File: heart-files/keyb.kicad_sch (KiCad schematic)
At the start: 180 parts, among them SW1 SW_Push, SW10 SW_Push, SW11 SW_Push, SW12 SW_Push, SW13 SW_Push, SW14 SW_Push, SW15 SW_Push, SW16 SW_Push, SW17 SW_Push, SW18 SW_Push, SW19 SW_Push, SW2 SW_Push, SW20 SW_Push, SW21 SW_Push, SW22 SW_Push, SW23 SW_Push, SW24 SW_Push, SW25 SW_Push, SW26 SW_Push, SW27 SW_Push, SW28 SW_Push, SW29 SW_Push, SW3 SW_Push, SW30 SW_Push, SW31 SW_Push, SW32 SW_Push, SW33 SW_Push, SW34 SW_Push, SW35 SW_Push, SW36 SW_Push, SW37 SW_Push, SW38 SW_Push, SW39 SW_Push, SW4 SW_Push, SW40 SW_Push, SW41 SW_Push, SW42 SW_Push, SW43 SW_Push, SW44 SW_Push, SW45 SW_Push, SW46 SW_Push, SW47 SW_Push, SW48 SW_Push, SW49 SW_Push, SW5 SW_Push, SW50 SW_Push, SW51 SW_Push, SW52 SW_Push, SW53 SW_Push, SW54 SW_Push, SW55 SW_Push, SW56 SW_Push, SW57 SW_Push, SW58 SW_Push, SW59 SW_Push, SW6 SW_Push, SW60 SW_Push, SW61 SW_Push, SW62 SW_Push, SW63 SW_Push, SW64 SW_Push, SW65 SW_Push, SW66 SW_Push, SW67 SW_Push, SW68 SW_Push, SW69 SW_Push, SW7 SW_Push, SW70 SW_Push, SW71 SW_Push, SW72 SW_Push, SW73 SW_Push, SW74 SW_Push, SW75 SW_Push, SW76 SW_Push, SW77 SW_Push, SW78 SW_Push, SW79 SW_Push, SW8 SW_Push, SW80 SW_Push, SW81 SW_Push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

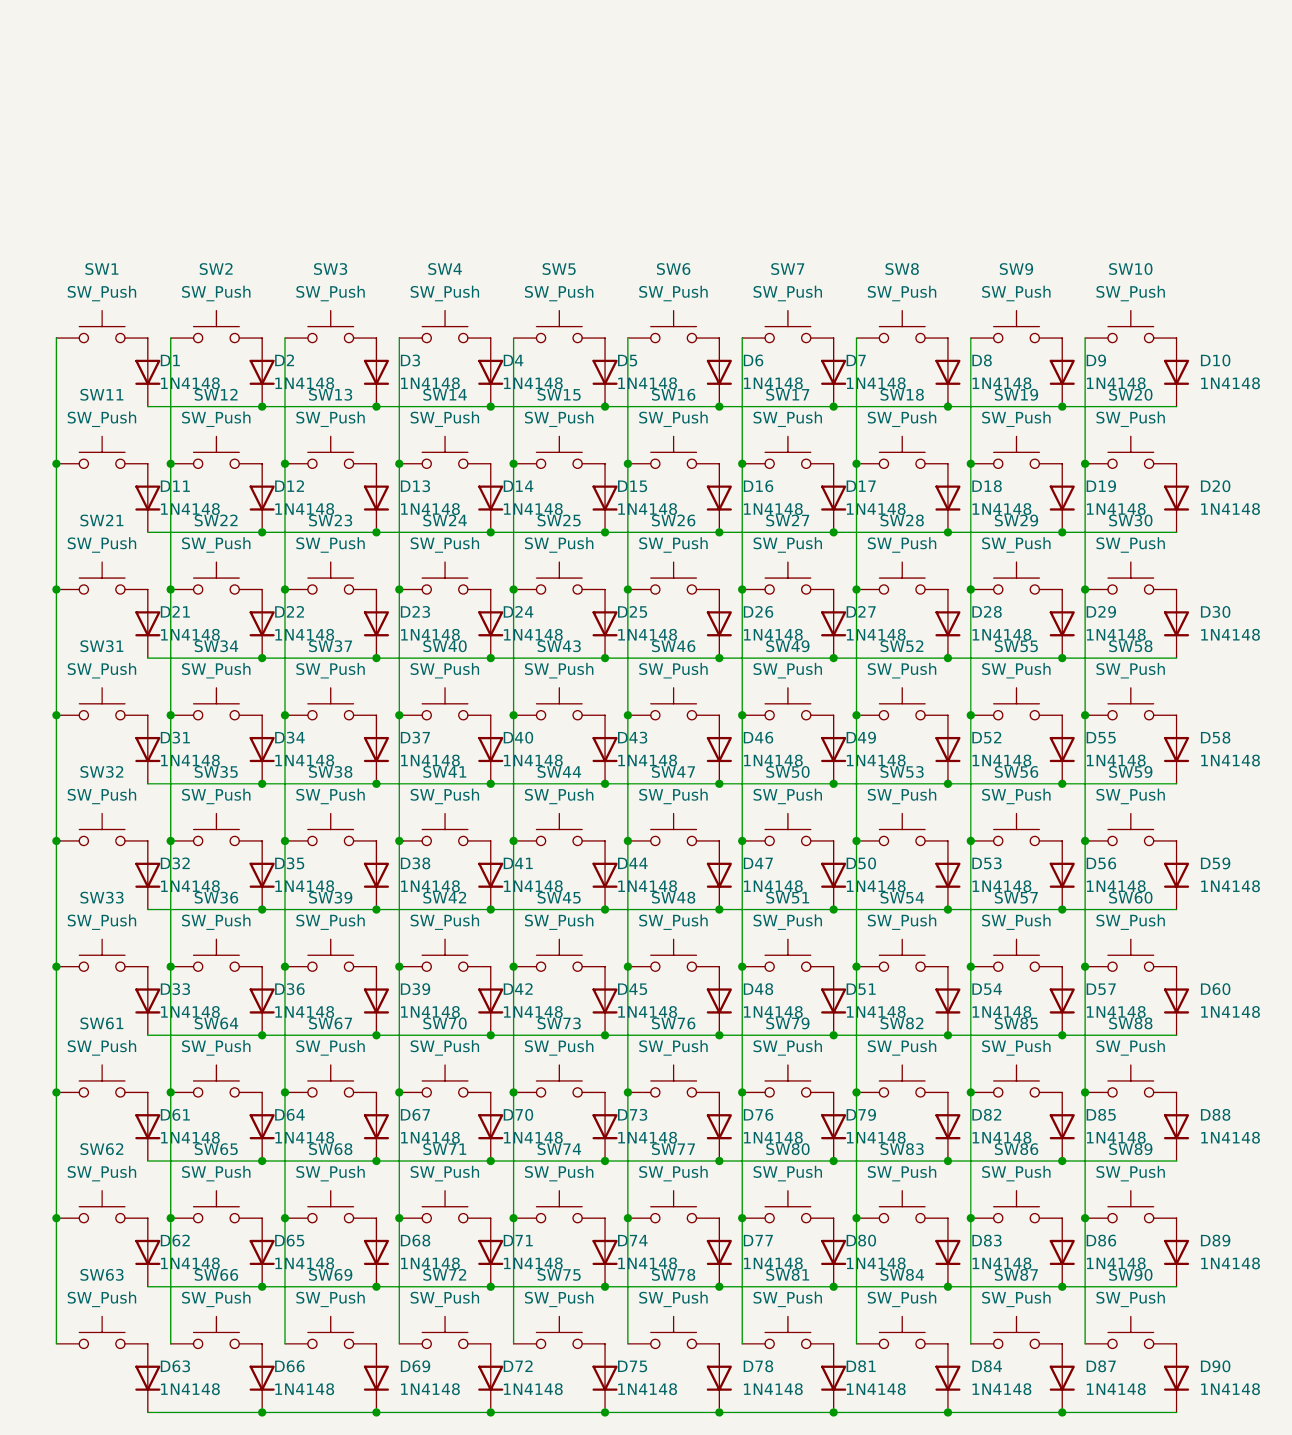
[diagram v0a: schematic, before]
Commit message: finished pcb, next is to review, document, push and submit
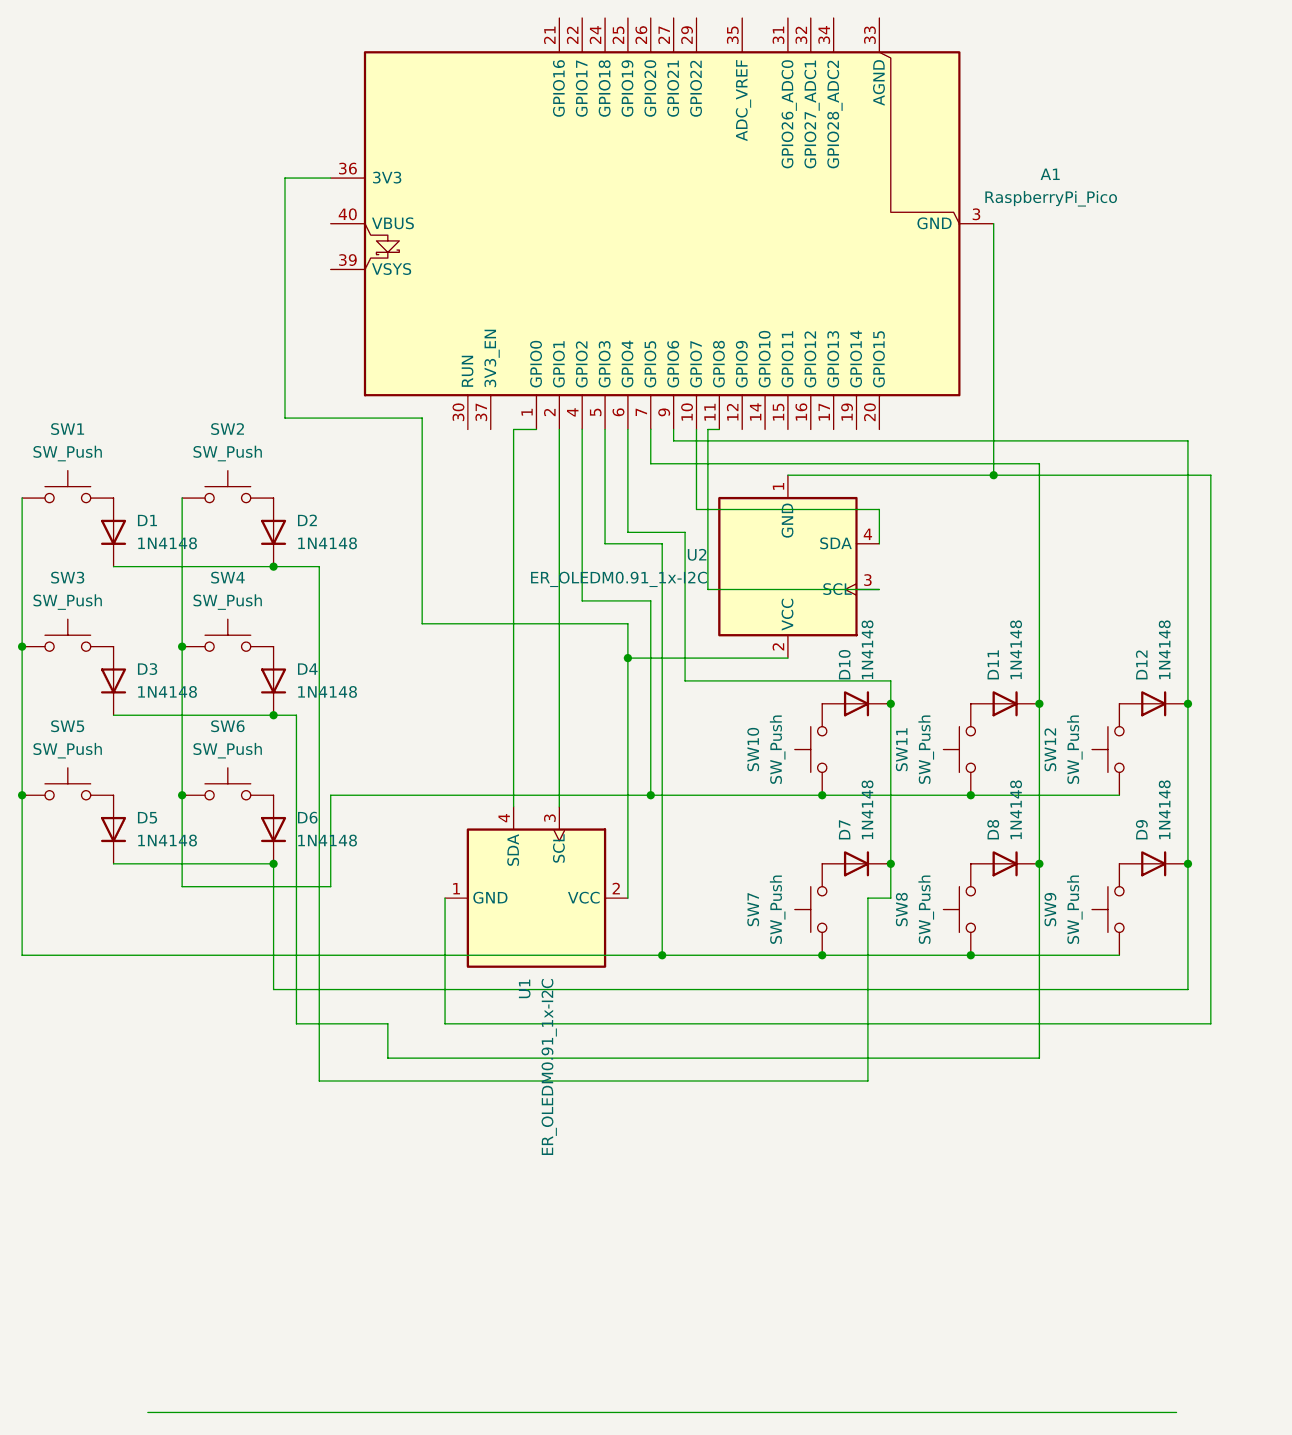
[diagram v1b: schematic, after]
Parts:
- removed D13, D14, D15, D16, D17, D18, D19, D20, D21, D22, D23, D24, D25, D26, D27, D28, D29, D30, D31, D32, D33, D34, D35, D36, D37, D38, D39, D40, D41, D42, D43, D44, D45, D46, D47, D48, D49, D50, D51, D52, D53, D54, D55, D56, D57, D58, D59, D60, D61, D62, D63, D64, D65, D66, D67, D68, D69, D70, D71, D72, D73, D74, D75, D76, D77, D78, D79, D80, D81, D82, D83, D84, D85, D86, D87, D88, D89, D90: 1N4148, Diode_THT:D_DO-35_SOD27_P7.62mm_Horizontal, symbol Diode:1N4148
- removed SW13, SW14, SW15, SW16, SW17, SW18, SW19, SW20, SW21, SW22, SW23, SW24, SW25, SW26, SW27, SW28, SW29, SW30, SW31, SW32, SW33, SW34, SW35, SW36, SW37, SW38, SW39, SW40, SW41, SW42, SW43, SW44, SW45, SW46, SW47, SW48, SW49, SW50, SW51, SW52, SW53, SW54, SW55, SW56, SW57, SW58, SW59, SW60, SW61, SW62, SW63, SW64, SW65, SW66, SW67, SW68, SW69, SW70, SW71, SW72, SW73, SW74, SW75, SW76, SW77, SW78, SW79, SW80, SW81, SW82, SW83, SW84, SW85, SW86, SW87, SW88, SW89, SW90: SW_Push, symbol Switch:SW_Push
- added A1: RaspberryPi_Pico, Module:RaspberryPi_Pico_Common_Unspecified, symbol MCU_Module:RaspberryPi_Pico
- added U1, U2: ER_OLEDM0.91_1x-I2C, Display:ER_OLEDM0.91_1x-I2C, symbol Display_Graphic:ER_OLEDM0.91_1x-I2C
- SW1, SW10, SW11, SW12, SW2, SW3, SW4, SW5, SW6, SW7, SW8, SW9: footprint (none) -> PCM_marbastlib-mx:SW_MX_1u
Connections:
- net at SW5.1: now also SW1.1, SW3.1, SW7.1, SW8.1, SW9.1, A1.5 (GPIO3)
- net at D12.1 (K): now also D5.1 (K), D6.1 (K), D9.1 (K), A1.9 (GPIO6); no longer D11.1 (K)
- net at SW10.1: now also SW11.1, SW12.1, SW2.1, SW4.1, SW6.1, A1.4 (GPIO2)
- new net: A1.13 (GND), A1.18 (GND), A1.23 (GND), A1.28 (GND), A1.3 (GND), A1.38 (GND), A1.8 (GND), U1.1 (GND), U2.1 (GND)
- new net: A1.36 (3V3), U1.2 (VCC), U2.2 (VCC)
- new net: A1.2 (GPIO1), U1.3 (SCL)
- new net: A1.1 (GPIO0), U1.4 (SDA)
- new net: A1.11 (GPIO8), U2.3 (SCL)
- new net: A1.10 (GPIO7), U2.4 (SDA)
- new net: A1.6 (GPIO4), D1.1 (K), D10.1 (K), D2.1 (K), D7.1 (K)
- new net: A1.7 (GPIO5), D11.1 (K), D3.1 (K), D4.1 (K), D8.1 (K)
